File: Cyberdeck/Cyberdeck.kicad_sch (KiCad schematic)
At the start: 22 parts, among them SW1 Slide Switch, U1 JST-PH BAT, U2 BQ24075 Charger, U3 0.47uH, U4 TPS62827 Regulator

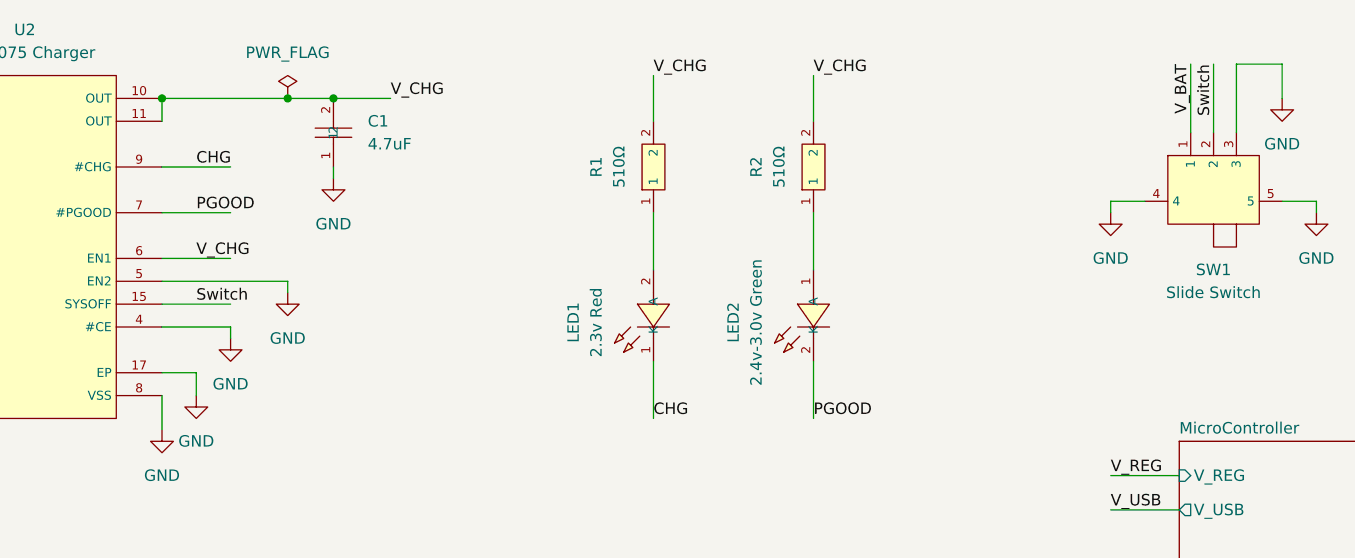
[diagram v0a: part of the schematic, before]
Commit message: Finalized PCB; Made gerber files
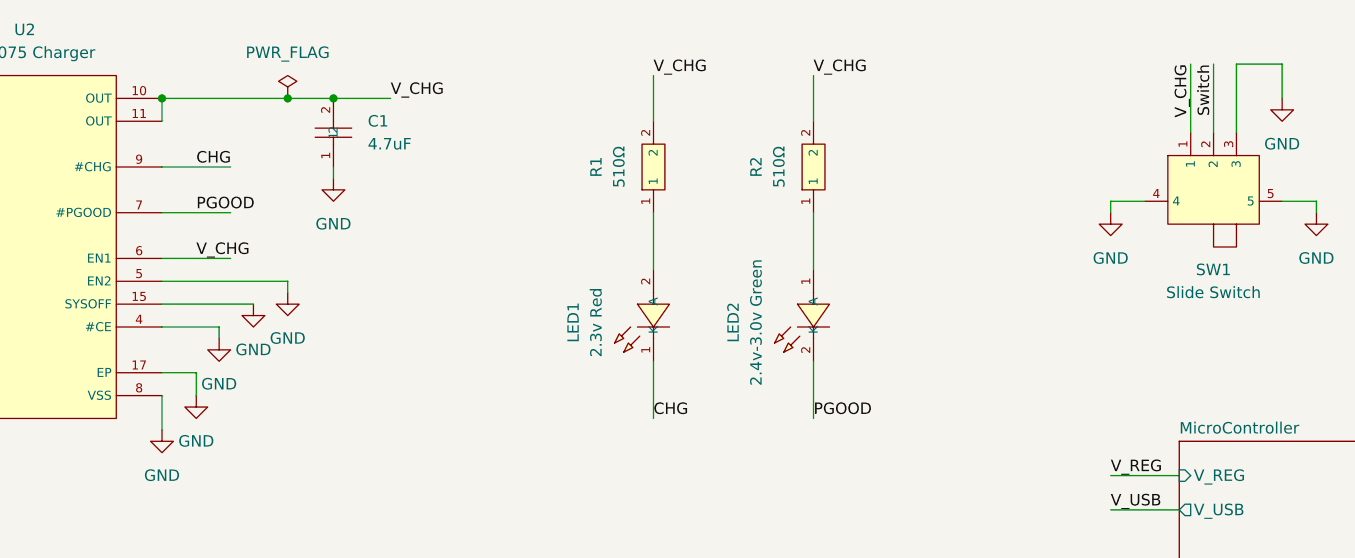
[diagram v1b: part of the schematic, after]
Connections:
- net GND: now also U2.15 (SYSOFF)
- net Switch: no longer U2.15 (SYSOFF)
- net V_BAT: no longer SW1.1
- net V_CHG: now also SW1.1
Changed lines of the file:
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@@
 	(wire
 		(pts
-			(xy 123.19 54.61) (xy 123.19 55.88)
+			(xy 121.92 54.61) (xy 121.92 55.88)
 		)
 		(stroke
@@
 	(wire
 		(pts
-			(xy 115.57 52.07) (xy 123.19 52.07)
+			(xy 115.57 52.07) (xy 125.73 52.07)
 		)
 		(stroke
@@
 	(wire
 		(pts
-			(xy 115.57 54.61) (xy 123.19 54.61)
+			(xy 115.57 54.61) (xy 121.92 54.61)
 		)
 		(stroke
@@
 		)
 	)
-	(label "V_BAT"
+	(label "V_CHG"
 		(at 229.87 25.4 270)
 		(effects
@@
 		)
 	)
-	(label "Switch"
-		(at 119.38 52.07 0)
-		(effects
-			(font
-				(size 1.27 1.27)
-			)
-			(justify left bottom)
-		)
-	)
 	(label "V_CHG"
 		(at 170.18 26.67 0)
@@
 		(dnp no)
 		(fields_autoplaced yes)
-		(property "Reference" "#PWR014"
+		(property "Reference" "#PWR017"
 			(at 90.17 138.43 0)
 			(hide yes)
@@
 			(project "Cyberdeck"
 				(path "/8993e48e-9b31-4221-b933-aeda00ea11c8"
-					(reference "#PWR014")
+					(reference "#PWR017")
 					(unit 1)
 				)
@@
 		(dnp no)
 		(fields_autoplaced yes)
-		(property "Reference" "#PWR053"
+		(property "Reference" "#PWR03"
 			(at 52.07 45.72 0)
 			(hide yes)
@@
 			(project "Cyberdeck"
 				(path "/8993e48e-9b31-4221-b933-aeda00ea11c8"
-					(reference "#PWR053")
+					(reference "#PWR03")
 					(unit 1)
 				)
@@
 		(dnp no)
 		(fields_autoplaced yes)
-		(property "Reference" "#PWR016"
+		(property "Reference" "#PWR019"
 			(at 57.15 176.53 0)
 			(hide yes)
@@
 			(project "Cyberdeck"
 				(path "/8993e48e-9b31-4221-b933-aeda00ea11c8"
-					(reference "#PWR016")
+					(reference "#PWR019")
 					(unit 1)
 				)
@@
 		(dnp no)
 		(fields_autoplaced yes)
-		(property "Reference" "#PWR015"
+		(property "Reference" "#PWR018"
 			(at 66.04 147.32 0)
 			(hide yes)
@@
 			(project "Cyberdeck"
 				(path "/8993e48e-9b31-4221-b933-aeda00ea11c8"
-					(reference "#PWR015")
+					(reference "#PWR018")
 					(unit 1)
 				)
@@
 		(dnp no)
 		(fields_autoplaced yes)
-		(property "Reference" "#PWR08"
+		(property "Reference" "#PWR011"
 			(at 119.38 68.58 0)
 			(hide yes)
@@
 			(project "Cyberdeck"
 				(path "/8993e48e-9b31-4221-b933-aeda00ea11c8"
-					(reference "#PWR08")
+					(reference "#PWR011")
 					(unit 1)
 				)
@@
 		(dnp no)
 		(fields_autoplaced yes)
-		(property "Reference" "#PWR054"
+		(property "Reference" "#PWR05"
 			(at 220.98 48.26 0)
 			(hide yes)
@@
 			(project "Cyberdeck"
 				(path "/8993e48e-9b31-4221-b933-aeda00ea11c8"
-					(reference "#PWR054")
+					(reference "#PWR05")
 					(unit 1)
 				)
@@
 		(dnp no)
 		(fields_autoplaced yes)
-		(property "Reference" "#PWR05"
+		(property "Reference" "#PWR07"
 			(at 129.54 57.15 0)
 			(hide yes)
@@
 			(project "Cyberdeck"
 				(path "/8993e48e-9b31-4221-b933-aeda00ea11c8"
-					(reference "#PWR05")
+					(reference "#PWR07")
 					(unit 1)
 				)
@@
 		(dnp no)
 		(fields_autoplaced yes)
-		(property "Reference" "#PWR09"
+		(property "Reference" "#PWR012"
 			(at 115.57 72.39 0)
 			(hide yes)
@@
 			(project "Cyberdeck"
 				(path "/8993e48e-9b31-4221-b933-aeda00ea11c8"
-					(reference "#PWR09")
+					(reference "#PWR012")
 					(unit 1)
 				)
@@
 		(dnp no)
 		(fields_autoplaced yes)
-		(property "Reference" "#PWR011"
+		(property "Reference" "#PWR014"
 			(at 73.66 87.63 0)
 			(hide yes)
@@
 			(project "Cyberdeck"
 				(path "/8993e48e-9b31-4221-b933-aeda00ea11c8"
-					(reference "#PWR011")
+					(reference "#PWR014")
 					(unit 1)
 				)
@@
 		(dnp no)
 		(fields_autoplaced yes)
-		(property "Reference" "#PWR010"
+		(property "Reference" "#PWR013"
 			(at 63.5 87.63 0)
 			(hide yes)
@@
 			(project "Cyberdeck"
 				(path "/8993e48e-9b31-4221-b933-aeda00ea11c8"
-					(reference "#PWR010")
+					(reference "#PWR013")
 					(unit 1)
 				)
@@
 		(dnp no)
 		(fields_autoplaced yes)
-		(property "Reference" "#PWR012"
+		(property "Reference" "#PWR015"
 			(at 85.09 87.63 0)
 			(hide yes)
@@
 			(project "Cyberdeck"
 				(path "/8993e48e-9b31-4221-b933-aeda00ea11c8"
-					(reference "#PWR012")
+					(reference "#PWR015")
 					(unit 1)
 				)
@@
 		(dnp no)
 		(fields_autoplaced yes)
-		(property "Reference" "#PWR04"
+		(property "Reference" "#PWR06"
 			(at 243.84 48.26 0)
 			(hide yes)
@@
 			(project "Cyberdeck"
 				(path "/8993e48e-9b31-4221-b933-aeda00ea11c8"
-					(reference "#PWR04")
+					(reference "#PWR06")
 					(unit 1)
 				)
@@
 	(symbol
 		(lib_id "power:GND")
+		(at 125.73 52.07 0)
+		(unit 1)
+		(body_style 1)
+		(exclude_from_sim no)
+		(in_bom yes)
+		(on_board yes)
+		(in_pos_files yes)
+		(dnp no)
+		(fields_autoplaced yes)
+		(property "Reference" "#PWR08"
+			(at 125.73 58.42 0)
+			(hide yes)
+			(show_name no)
+			(do_not_autoplace no)
+			(effects
+				(font
+					(size 1.27 1.27)
+				)
+			)
+		)
+		(property "Value" "GND"
+			(at 125.73 57.15 0)
+			(show_name no)
+			(do_not_autoplace no)
+			(effects
+				(font
+					(size 1.27 1.27)
+				)
+			)
+		)
+		(property "Footprint" ""
+			(at 125.73 52.07 0)
+			(hide yes)
+			(show_name no)
+			(do_not_autoplace no)
+			(effects
+				(font
+					(size 1.27 1.27)
+				)
+			)
+		)
+		(property "Datasheet" ""
+			(at 125.73 52.07 0)
+			(hide yes)
+			(show_name no)
+			(do_not_autoplace no)
+			(effects
+				(font
+					(size 1.27 1.27)
+				)
+			)
+		)
+		(property "Description" "Power symbol creates a global label with name \"GND\" , ground"
+			(at 125.73 52.07 0)
+			(hide yes)
+			(show_name no)
+			(do_not_autoplace no)
+			(effects
+				(font
+					(size 1.27 1.27)
+				)
+			)
+		)
+		(pin "1"
+		)
+		(instances
+			(project "Cyberdeck"
+				(path "/8993e48e-9b31-4221-b933-aeda00ea11c8"
+					(reference "#PWR08")
+					(unit 1)
+				)
+			)
+		)
+	)
+	(symbol
+		(lib_id "power:GND")
 		(at 66.04 40.64 0)
 		(unit 1)
@@
 		(dnp no)
 		(fields_autoplaced yes)
-		(property "Reference" "#PWR03"
+		(property "Reference" "#PWR04"
 			(at 66.04 46.99 0)
 			(hide yes)
@@
 			(project "Cyberdeck"
 				(path "/8993e48e-9b31-4221-b933-aeda00ea11c8"
-					(reference "#PWR03")
+					(reference "#PWR04")
 					(unit 1)
 				)
@@
 		(dnp no)
 		(fields_autoplaced yes)
-		(property "Reference" "#PWR07"
+		(property "Reference" "#PWR010"
 			(at 60.96 63.5 0)
 			(hide yes)
@@
 			(project "Cyberdeck"
 				(path "/8993e48e-9b31-4221-b933-aeda00ea11c8"
-					(reference "#PWR07")
+					(reference "#PWR010")
 					(unit 1)
 				)
@@
 	(symbol
 		(lib_id "power:GND")
-		(at 123.19 55.88 0)
+		(at 121.92 55.88 0)
 		(unit 1)
 		(body_style 1)
@@
 		(dnp no)
 		(fields_autoplaced yes)
-		(property "Reference" "#PWR06"
-			(at 123.19 62.23 0)
+		(property "Reference" "#PWR09"
+			(at 121.92 62.23 0)
 			(hide yes)
 			(show_name no)
@@
 		)
 		(property "Value" "GND"
-			(at 123.19 60.96 0)
+			(at 121.92 60.96 0)
 			(show_name no)
 			(do_not_autoplace no)
@@
 		)
 		(property "Footprint" ""
-			(at 123.19 55.88 0)
+			(at 121.92 55.88 0)
 			(hide yes)
 			(show_name no)
@@
 		)
 		(property "Datasheet" ""
-			(at 123.19 55.88 0)
+			(at 121.92 55.88 0)
 			(hide yes)
 			(show_name no)
@@
 		)
 		(property "Description" "Power symbol creates a global label with name \"GND\" , ground"
-			(at 123.19 55.88 0)
+			(at 121.92 55.88 0)
 			(hide yes)
 			(show_name no)
@@
 			(project "Cyberdeck"
 				(path "/8993e48e-9b31-4221-b933-aeda00ea11c8"
-					(reference "#PWR06")
+					(reference "#PWR09")
 					(unit 1)
 				)
@@
 		(dnp no)
 		(fields_autoplaced yes)
-		(property "Reference" "#PWR013"
+		(property "Reference" "#PWR016"
 			(at 134.62 137.16 0)
 			(hide yes)
@@
 			(project "Cyberdeck"
 				(path "/8993e48e-9b31-4221-b933-aeda00ea11c8"
-					(reference "#PWR013")
+					(reference "#PWR016")
 					(unit 1)
 				)
